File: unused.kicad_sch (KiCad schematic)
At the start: 4 parts, among them U2 74LS08, U3 74LS32, U4 74LS02, U6 NE556

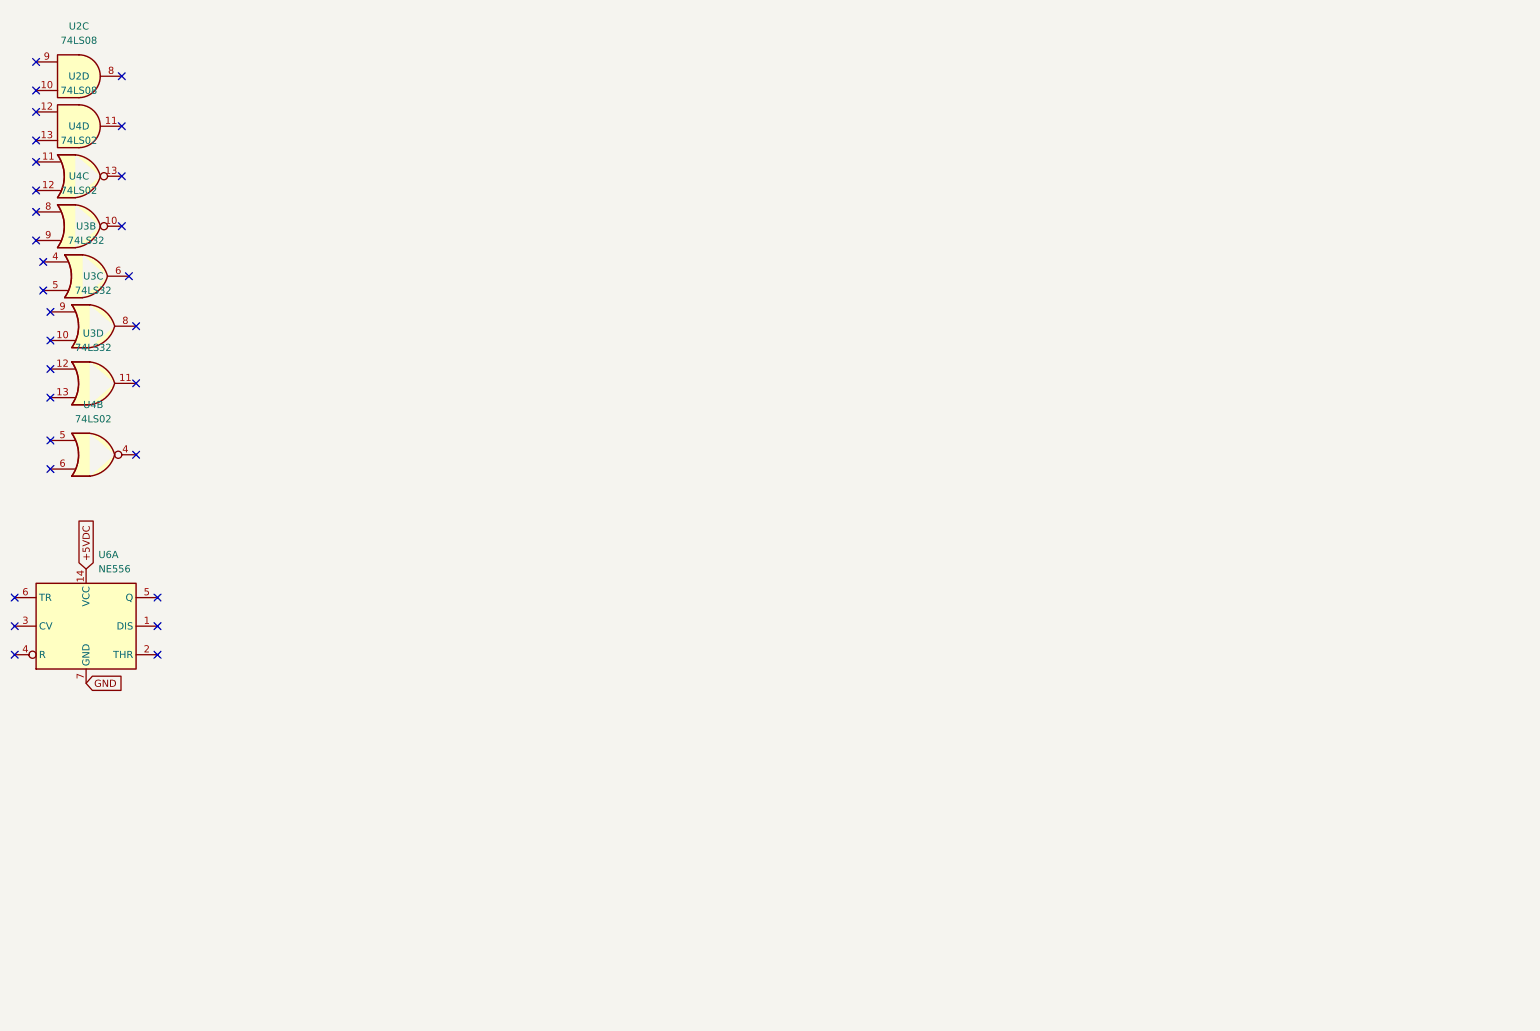
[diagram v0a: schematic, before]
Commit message: Add files via upload
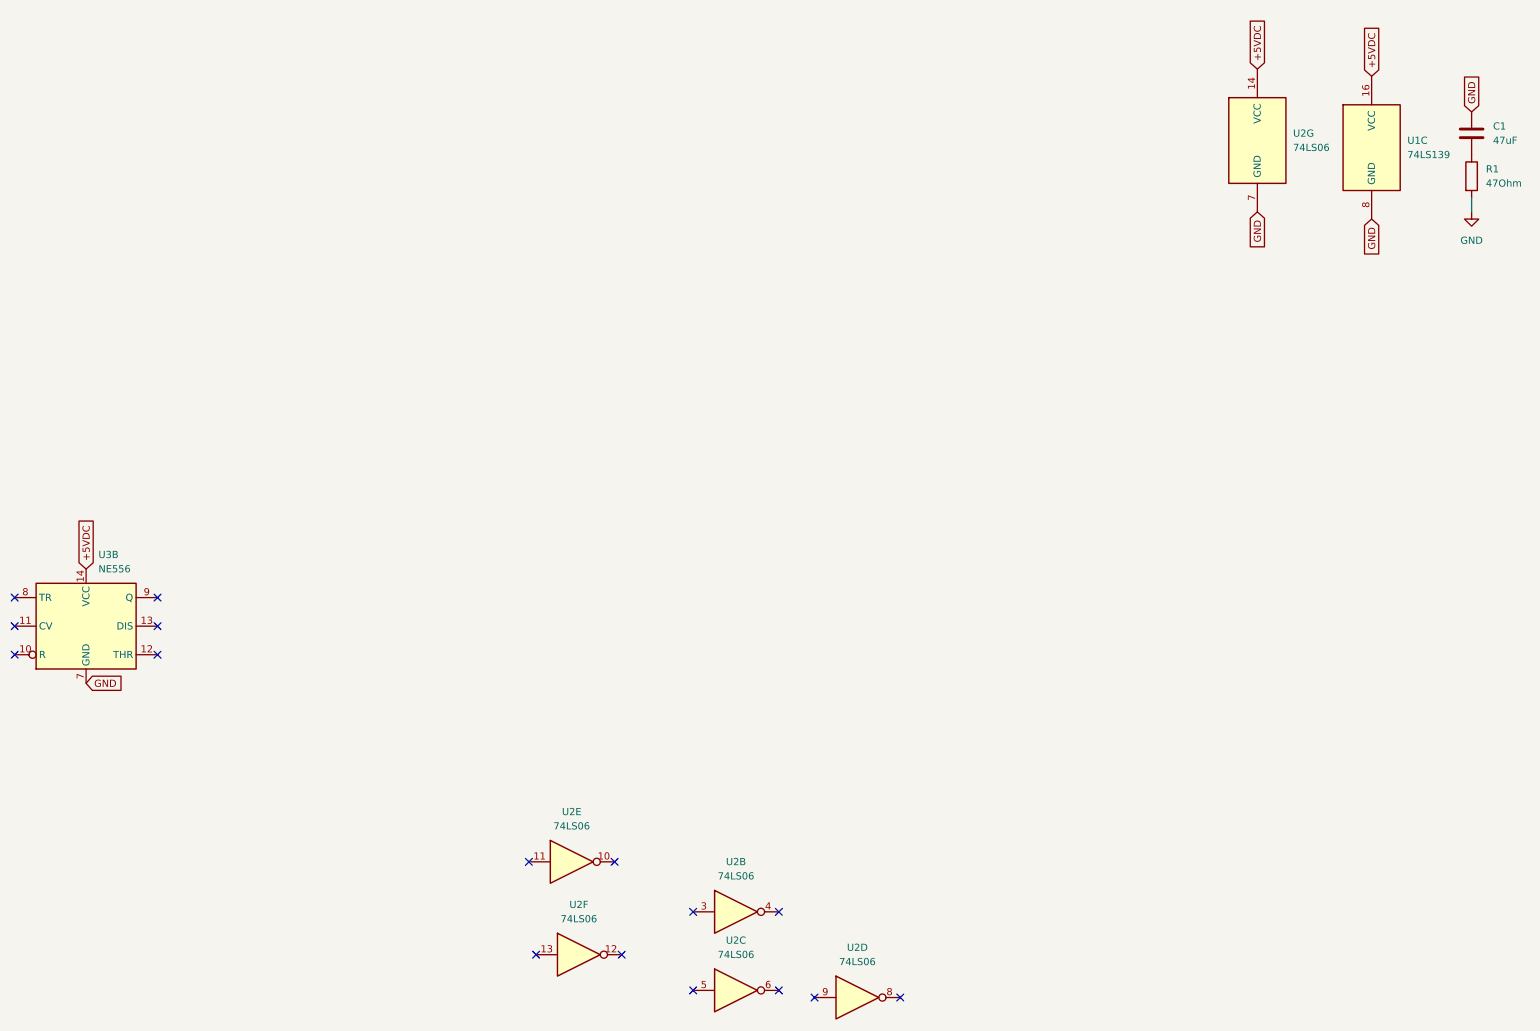
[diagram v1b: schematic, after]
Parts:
- removed U2: 74LS08, symbol 74xx:74LS08
- removed U3: 74LS32, Package_DIP:DIP-14_W7.62mm_LongPads, symbol 74xx:74LS32
- removed U4: 74LS02, Package_DIP:DIP-14_W7.62mm_LongPads, symbol 74xx:74LS02
- added C1: 47uF, Capacitor_THT:C_Disc_D9.0mm_W5.0mm_P7.50mm, symbol Device:C
- added R1: 47Ohm, Resistor_THT:R_Axial_DIN0411_L9.9mm_D3.6mm_P7.62mm_Vertical, symbol Device:R
- added U1: 74LS139, symbol 74xx:74LS139
- added U2: 74LS06, Package_DIP:DIP-14_W7.62mm_LongPads, symbol 74xx:74LS06
- renumbered U6 to U3
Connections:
- net +5VDC: now also U1.16 (VCC), U2.14 (VCC)
- net GND: now also C1.1, R1.2, U1.8 (GND), U2.7 (GND)
- new net: C1.2, R1.1
- no-connect marks 30 -> 16
